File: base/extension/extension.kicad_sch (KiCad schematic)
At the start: 23 parts, among them J1 USB_C_Receptacle_USB2.0_16P, J2 Conn_02x20_Odd_Even, J3 2-1734248-0, J4 Conn_01x02, J5 2-1734248-0, J9 610 mm ffc cable, U1 LM7805_TO263, U2 MCP1700T-3302E/TT, U3 CH224K

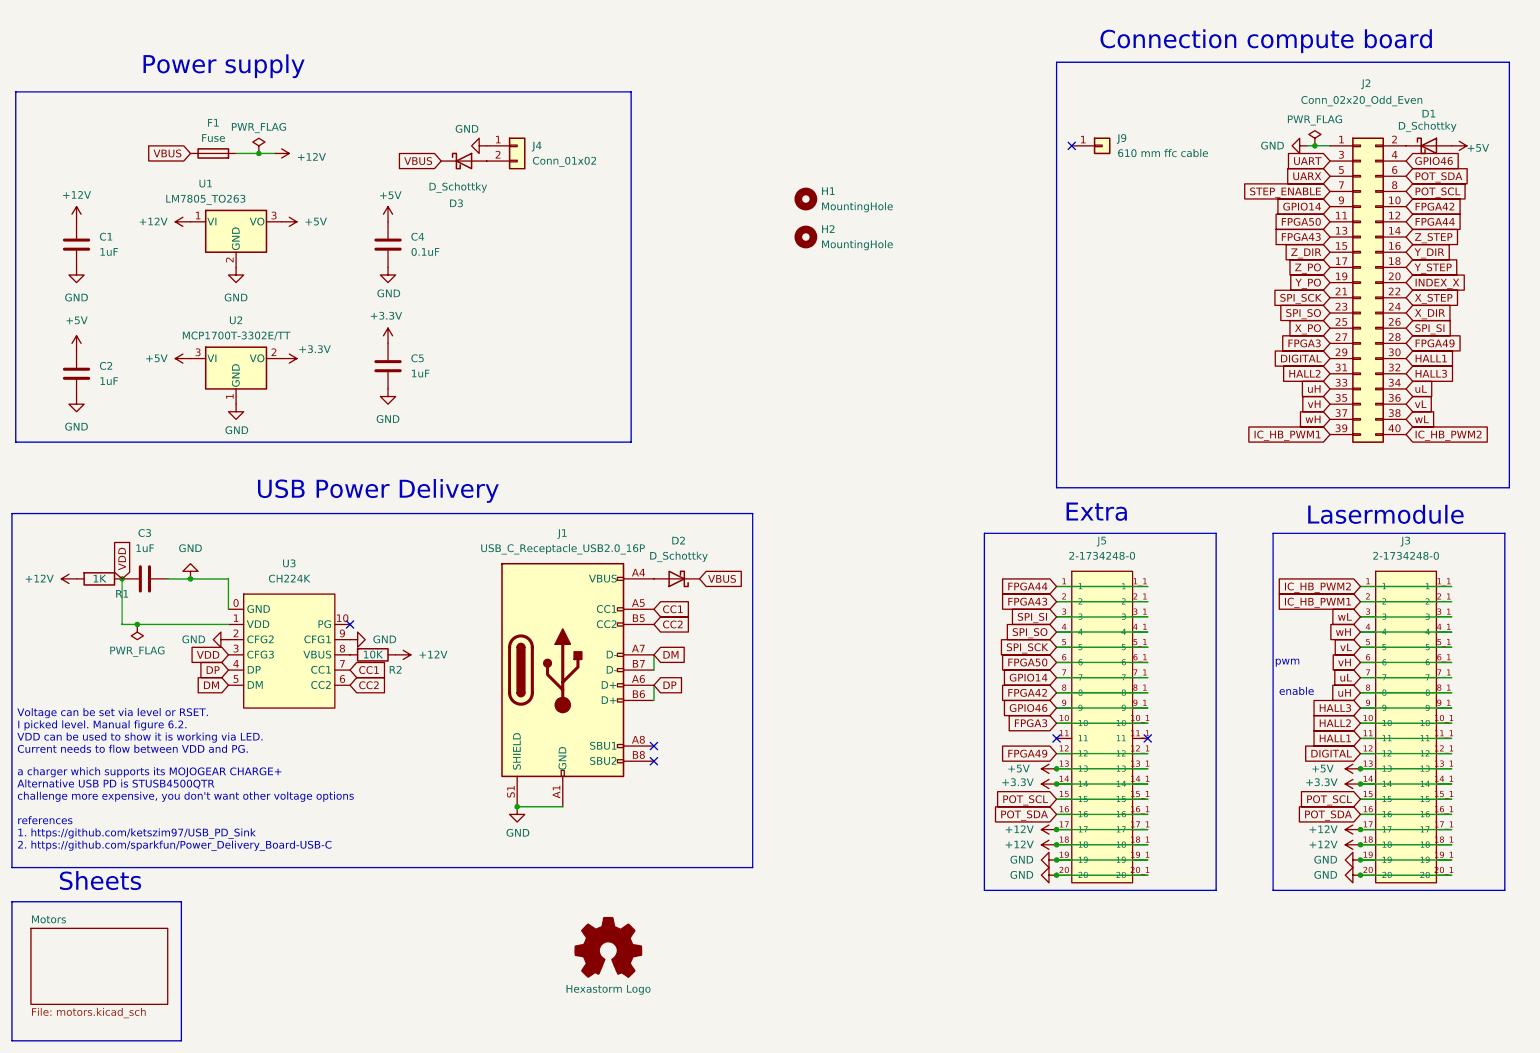
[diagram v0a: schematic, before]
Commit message: schema  extension finished, pre  merge
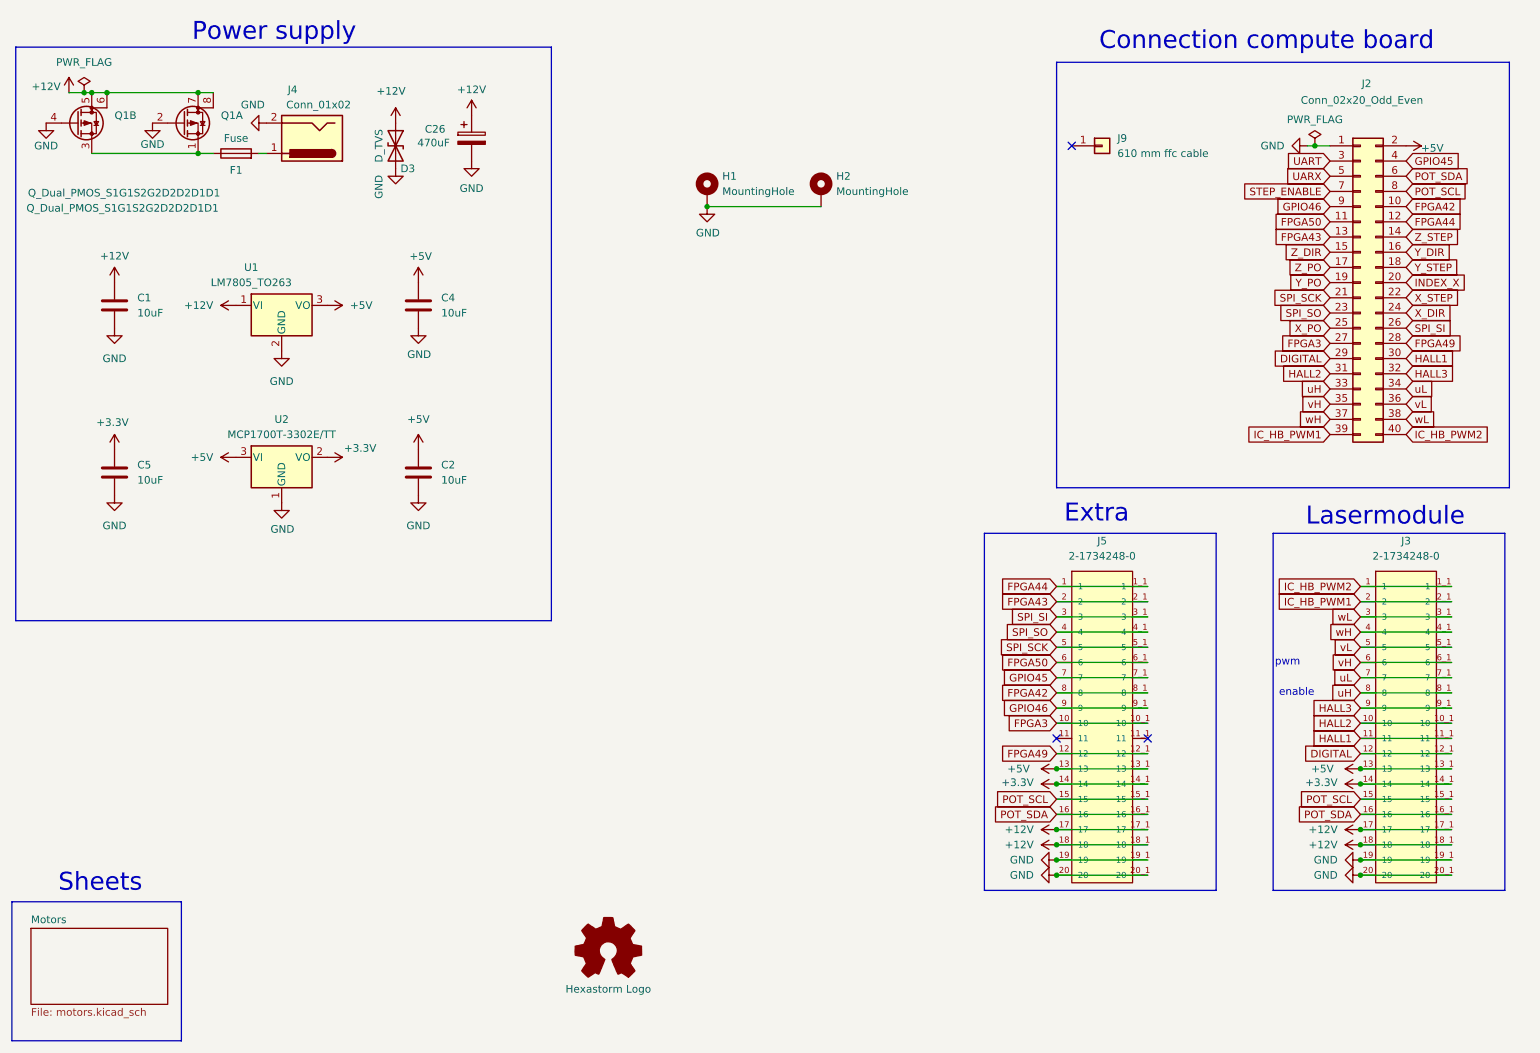
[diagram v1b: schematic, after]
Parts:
- removed C3: 1uF, Capacitor_SMD:C_0805_2012Metric_Pad1.18x1.45mm_HandSolder, symbol Device:C
- removed D1, D2: D_Schottky, Diode_SMD:D_SMA, symbol Device:D_Schottky
- removed J1: USB_C_Receptacle_USB2.0_16P, footprints:USB_C_Receptacle_GCT_USB4105-xx-A_16P_TopMnt_Horizontal, symbol Connector:USB_C_Receptacle_USB2.0_16P
- removed R1: 1K, Resistor_SMD:R_0805_2012Metric, symbol Device:R
- removed R2: 10K, Resistor_SMD:R_0805_2012Metric, symbol Device:R
- removed U3: CH224K, footprints:ESSOP-10_CH224K, symbol wch_mcu_peripheral:CH224K
- added C26: 470uF, Capacitor_SMD:CP_Elec_10x10.5, symbol Device:C_Polarized
- added Q1: Q_Dual_PMOS_S1G1S2G2D2D2D1D1, Package_SO:SOIC-8_3.9x4.9mm_P1.27mm, symbol Transistor_FET:Q_Dual_PMOS_S1G1S2G2D2D2D1D1
- C1, C5: value 1uF -> 10uF; Farnell 2094043 -> (none); farnell# 2094043 -> CL21A106KAYNNNE; manf# 08055C105KAT2A -> 187-CL21A106KAYNNNE; mouser# 581-08055C105KAT2A -> 3010126
- C2: value 1uF -> 10uF; farnell# 2094043 -> CL21A106KAYNNNE; manf# 08055C105KAT2A -> 187-CL21A106KAYNNNE; mouser# 581-08055C105KAT2A -> 3010126
- C4: value 0.1uF -> 10uF; Farnell 1414663 -> (none); farnell# 1414663 -> CL21A106KAYNNNE; manf# C0805C104J5RACTU -> 187-CL21A106KAYNNNE; mouser# 80-C0805C104J5R -> 3010126
- D3: value D_Schottky -> D_TVS; footprint Diode_SMD:D_SMA -> Diode_SMD:D_SMB; symbol Device:D_Schottky -> Device:D_TVS; farnell# 2335183 -> 2765106; manf# B340A-E3/61T -> SMBJ13CA; mouser# 625-BD340A-E3/61T -> 652-SMBJ13CA
- F1: footprint Fuse:Fuse_0603_1608Metric_Pad1.05x0.95mm_HandSolder -> Fuse:Fuse_2920_7451Metric; farnell# 2799441 -> 2336373; manf# SF-1206FP500-2 -> MF-LSMF300/24X-2; mouser# 652-SF-1206FP500-2 -> 652-MF-LSMF300/24X-2
- H1, H2: footprint MountingHole:MountingHole_2.2mm_M2 -> MountingHole:MountingHole_2.2mm_M2_Pad_Via; symbol Mechanical:MountingHole -> Mechanical:MountingHole_Pad; now left out of the parts list
- J2: mouser# (none) -> 649-221121-00040T4LF
- J3, J5: farnell# (none) -> 3404513
- J4: footprint footprints:VN02A1500000G -> Connector_BarrelJack:BarrelJack_CUI_PJ-036AH-SMT_Horizontal; symbol Connector_Generic:Conn_01x02 -> Connector:Jack-DC; Farnell 3817460 -> (none); farnell# (none) -> 4814431; manf# VN02A1500000G -> PJ-036AH-SMT-TR; mouser# 649-VN02A15000J0G -> 490-PJ-036AH-SMT-TR
- J9: mouser# (none) -> 538-15167-0361
- U1: farnell# (none) -> 2102566
- U2: farnell# (none) -> 1296592
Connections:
- net +12V: now also D3.1 (A1), C26.1, Q1.5 (D), Q1.6 (D), Q1.7 (D), Q1.8 (D); no longer F1.2
- net +5V: now also J2.2 (Pin_2)
- net GND: now also D3.2 (A2), H1.1, H2.1, J4.2, C26.2, Q1.2 (G), Q1.4 (G); no longer J4.1 (Pin_1)
- net GPIO46: now also J2.9 (Pin_9); no longer J2.4 (Pin_4)
- net GPIO14 renamed GPIO45
- net GPIO45: now also J2.4 (Pin_4); no longer J2.9 (Pin_9)
- net VBUS: no longer names the net of F1.1
- net VBUS: now also Q1.1 (S), Q1.3 (S); no longer D3.1 (K)
- new net: F1.2, J4.1
- no-connect marks 6 -> 3
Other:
- note removed: "USB Power Delivery"
- note removed: "Voltage can be set via level or RSET. I picked level. Manual figure 6.2. VDD can be used to show it is working via LED. Current needs to flow between VDD and PG."
- note removed: "a charger which supports its MOJOGEAR CHARGE+ Alternative USB PD is STUSB4500QTR challenge more expensive, you don't want other voltage options references 1. https://github.com/ketszim97/USB_PD_Sink 2. https://github.com/sparkfun/Power_Delivery_Board-USB-C"
- moved on the sheet: C1, C2, C4, C5, D3, F1, U1, U2
